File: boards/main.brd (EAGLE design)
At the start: 100 x 65 mm, 195 parts, among them IC1 24AA32ASN, IC2 INA194, IC3 LP2950Z, Q1 IRLML5203, Q2 IRLML5103, T3 BC848, U1 ITG-3200, U2 TMP75DGK, U3 MAG3110, U4 MMA8451Q, U44 BMP085, U5 MAX1236EUA+, X1 USB-SMD-NS

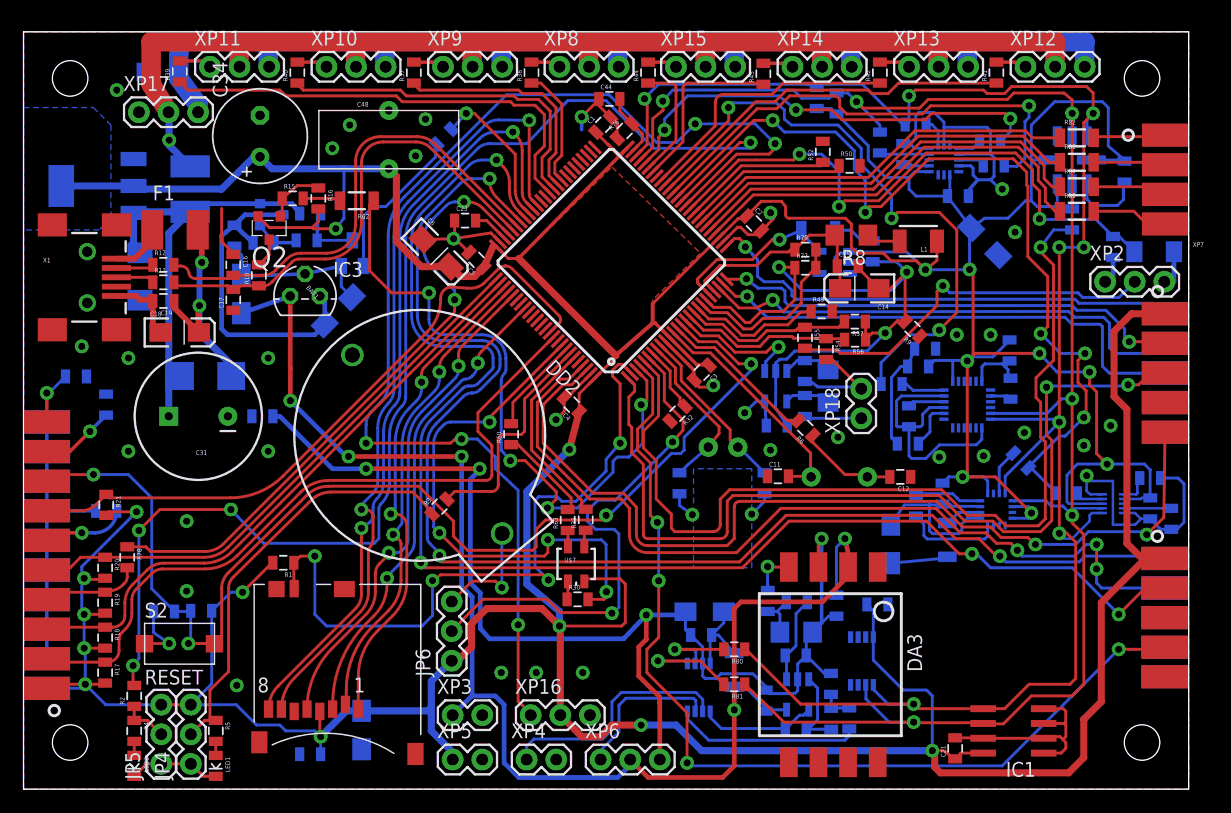
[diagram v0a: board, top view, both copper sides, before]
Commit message: put all the downloaded files into directories
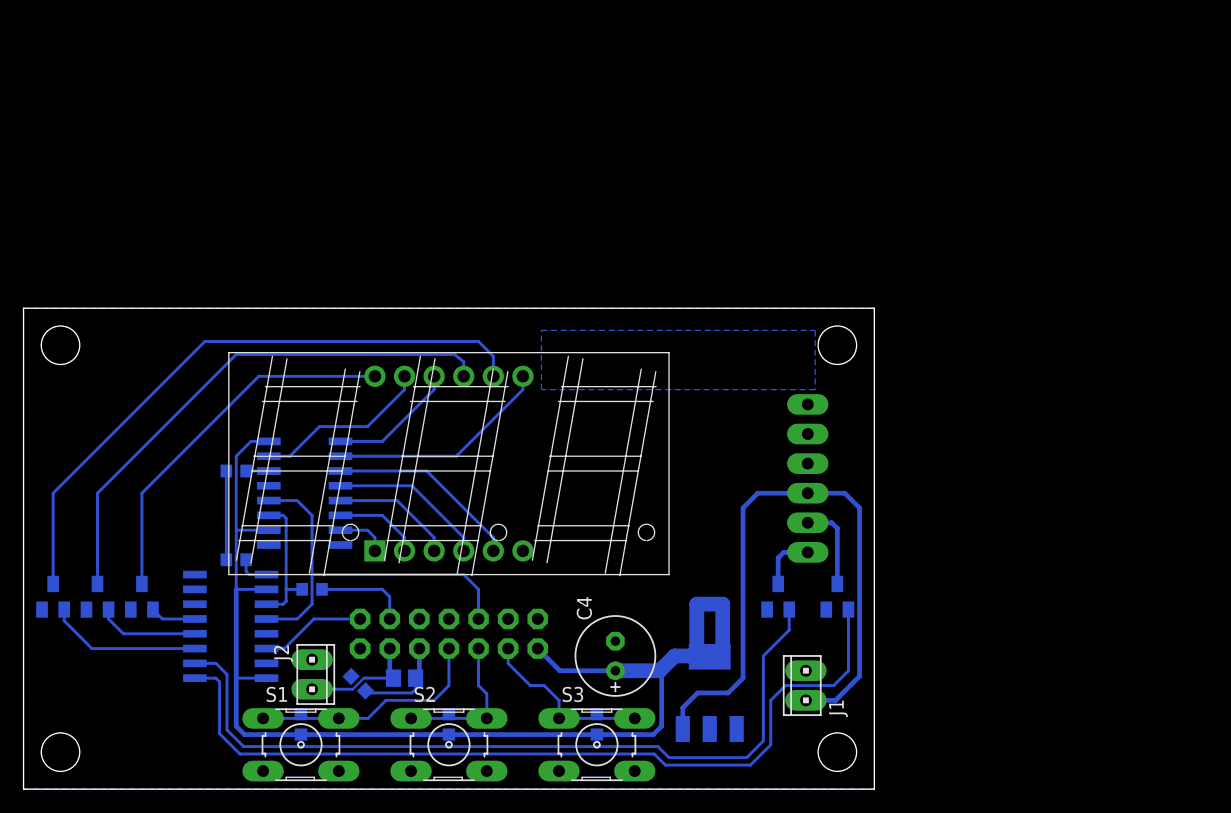
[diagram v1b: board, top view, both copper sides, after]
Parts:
- removed BAT1: 3V, SparkFun:BATTCOM_20MM_PTH
- removed C10, C9: 10pF, SparkFun:0805
- removed C11, C12, C16, C17: 20pF, SparkFun:0805
- removed C13, C15, C19, C20, C21, C22, C24, C25, C27, C28, C29, C32, C33, C36, C37, C38, C42, C43, C50, C54, C55, C8: 0.1uF, SparkFun:0805
- removed C14, C18, C52, C6: 10uF/6.3v, SparkFun:EIA3216-KIT
- removed C23, C44: 2.2uF, SparkFun:0805
- removed C26, C35, C41: 4.7uF, SparkFun:EIA3216-KIT
- removed C30: 1uF, SparkFun:0805
- removed C31: 330uF/16v, SparkFun:CPOL-RADIAL-1000UF-25V
- removed C34: 560uF/4v, rcl:E3,5-8
- removed C39: 2.2nF/50v, SparkFun:0805
- removed C40: 0.22uF, SparkFun:0805
- removed C45: 10uF, SparkFun:1206
- removed C48: 0.22F/5.5v, barthess:CAP-IONISTOR-5MM
- removed C49: 2.2uF, rcl:C1206
- removed C51: 10uF/16v, SparkFun:EIA3216-KIT
- removed C7: 47uF/6.3v, SparkFun:EIA3216-KIT
- removed D2: 10BQ060, diode:SMB
- removed D3: SM6T12V, diode:SMBJ
- removed DA1: LM1117, barthess:SOT223
- removed DA2: LMV321M5, linear:SOT23-5
- removed DA3: MPXV5010DP, barthess:482
- removed DA6: LP2980, barthess:SOT23-5
- removed DD1: MICROSD_SDIO, barthess:MICROSD
- removed DD2: STM32F103VDT6, barthess:TQFP100
- removed DD3: HMC5883L, barthess:16LPCC
- removed F1, F3: POLYSWITCH, barthess:1812
- removed IC2: INA194, barthess:SOT23-5
- removed JP1: 2X5, barthess:2X5-PSEUDOSMD
- removed JP3, JP7, JP8, JP9: STAND-OFFTIGHT, SparkFun:STAND-OFF-TIGHT
- removed JP4: boot_0, SparkFun:1X03
- removed JP5: boot_1, SparkFun:1X03
- removed JP6: bat, SparkFun:1X03
- removed L1: 1uH, SparkFun:1210
- removed LED1, LED2: RED, barthess:LED-0805
- removed R10, R35: 1.5k, SparkFun:0805
- removed R12, R13: 33, SparkFun:0805
- removed R15, R27, R28: 2.7k, SparkFun:0805
- removed R16, R17, R18, R19, R20, R21, R22, R23, R24, R45, R48, R54, R55, R59, R7: 10k, SparkFun:0805
- removed R25, R53: 2.2, barthess:R1206
- removed R26: 1, SparkFun:0805
- removed R29, R46, R56, R57, R58, R61, R66, R67, R69, R71, R72, R75: 1k, SparkFun:0805
- removed R30, R63: 68, SparkFun:0805
- removed R31, R60, R65, R70, R73, R74, R76, R77, R78, R79, R80, R81, R9: 0, SparkFun:0805
- removed R32, R33, R47: 100k, SparkFun:0805
- removed R34: 30k, SparkFun:0805
- removed R36, R51: 47, SparkFun:0805
- removed R37, R38, R39, R40, R41, R42, R43, R44, R49, R50, R52, R6: 330, SparkFun:0805
- removed R5: 100, SparkFun:0805
- removed R62, R64, R68, R82, R83, R84, R85: 0, barthess:R1206
- removed R8: 2.2, rcl:R1206
- removed T3: BC848, transistor:SOT23
- removed U$7: LED-TRICOLOR, SparkFun:LED-TRICOLOR-SMD
- removed U1: ITG-3200, barthess:QFN-24
- removed U2: TMP75DGK, barthess:MSOP8
- removed U3: MAG3110, barthess:DFN-10
- removed U4: MMA8451Q, barthess:QFN-16_0.5MM
- removed U44: BMP085, barthess:BMP085
- removed U5: MAX1236EUA+, barthess:MSOP8
- removed VD8: BZV55-C3V3, barthess:SOD80C
- removed X1: USB-SMD-NS, SparkFun:USB-MINIB-NOSTOP
- removed XP1: 2X10-PSEUDO_SMD, barthess:2X10-PSEUDOSMD
- removed XP10: PWM3, SparkFun:1X03
- removed XP11: PWM4, SparkFun:1X03
- removed XP12: PWM5, SparkFun:1X03
- removed XP13: PWM6, SparkFun:1X03
- removed XP14: PWM7, SparkFun:1X03
- removed XP15: PWM8, SparkFun:1X03
- removed XP16: tacho, SparkFun:1X03
- removed XP17: power, SparkFun:1X03
- removed XP18: current_sens, barthess:1X02
- removed XP2: RECEIVER, SparkFun:1X03
- removed XP3: EXT_5V, barthess:1X02
- removed XP4: an2_5v, barthess:1X02
- removed XP5: EXT3.3V, barthess:1X02
- removed XP6: sonar, SparkFun:1X03
- removed XP7: SPI_EXT, barthess:1X4-PSEUDOSMD
- removed XP8: PWM1, SparkFun:1X03
- removed XP9: PWM2, SparkFun:1X03
- removed ZQ1: 8M, barthess:HC49U-V
- removed ZQ2: 32k, barthess:TC38H
- added 430: (no value), pinhead:2X07
- added IC4: 74LS595D, 74xx-us:SO16
- added J1, J2: (no value), con-amp:10X02MTA
- added Q3, Q4, Q5: BSS123, transistor-small-signal:SOT23
- added S1, S3: (no value), switch-omron:B3F-10XX
- added U$1: BL-T52C-31, mjg:BL-T52X-31
- C1, C2, C3: value 0.1uF -> (none); device SparkFun:0805 -> rcl:C0603K
- C4: value 0.1uF -> (none); device SparkFun:0805 -> rcl:E2,5-7
- C5: value 0.1uF -> 470nF; device SparkFun:0805 -> rcl:C0603K
- IC1: value 24AA32ASN -> 74LS595D; device barthess:SO-08 -> 74xx-us:SO16
- IC3: value LP2950Z -> 317EMP; device linear:TO92 -> linear:SOT223
- JP2: value 2X5 -> (none); device barthess:2X5-PSEUDOSMD -> pinhead:1X06
- Q1: value IRLML5203 -> BSS123; device transistor-power:MICRO3 -> transistor-small-signal:SOT23
- Q2: value IRLML5103 -> BSS123; device transistor-power:MICRO3 -> transistor-small-signal:SOT23
- R1, R2: value 10k -> 0; device SparkFun:0805 -> rcl:R0603
- R3: value 10k -> 720ish; device SparkFun:0805 -> rcl:R0805
- R4: value 100 -> 0; device SparkFun:0805 -> rcl:R0603
- S2: value RESET -> (none); device barthess:BUTTON_6X3.5 -> switch-omron:B3F-10XX
- moved IC1 67.8 mm to (17.8, 14.0), flipped to the bottom
- moved C1 51.5 mm to (49.2, 5.56), flipped to the bottom, turned to 270 degrees
- moved C2 50.3 mm to (36.5, 5.56), flipped to the bottom, turned to 270 degrees
- moved IC3 48.7 mm to (58.9, 8.26), flipped to the bottom
- moved C3 45.8 mm to (23.8, 5.56), flipped to the bottom, turned to 270 degrees
- moved Q1 37.8 mm to (2.54, 16.5), turned to 0 degrees
- moved C5 37.8 mm to (28.7, 9.05), flipped to the bottom, turned to 225 degrees
- moved Q2 34.9 mm to (6.35, 16.5), flipped to the bottom, turned to 0 degrees
- moved JP2 32.9 mm to (67.3, 26.7), flipped to the bottom, turned to 270 degrees
- moved S2 28.1 mm to (36.5, 3.81)
- moved C4 21.9 mm to (50.8, 11.4), turned to 90 degrees
- moved R2 21.2 mm to (18.3, 27.3), flipped to the bottom, turned to 180 degrees
- moved R4 19.5 mm to (24.8, 17.1), flipped to the bottom, turned to 0 degrees
- moved R3 15.0 mm to (32.7, 9.53), flipped to the bottom, turned to 180 degrees
- moved R1 4.05 mm to (18.3, 19.7), flipped to the bottom, turned to 0 degrees
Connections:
- removed net 3.3V: C1.1, C2.1, C20.1, C21.1, C27.2, C3.1, C30.1, C33.2, C34.+, C35.A, C37.2, C4.1, C42.1, C48.1, C5.1, C6.A, C7.A, C8.2, DA1.2, DA1.4, DA6.1, DA6.3, DD1.4, DD2.100, DD2.11, DD2.28, DD2.50, DD2.75, DD3.13, DD3.2, DD3.4, IC1.8, JP1.1, JP2.1, JP4.3, JP5.3, JP6.1, L1.1, Q2.2, R1.2, R16.2, R17.2, R18.2, R19.2, R20.2, R21.2, R26.2, R27.2, R28.2, R7.2, U$7.A, U1.13, U2.8, U3.2, U3.8, U4.1, U4.14, U44.3, U44.4, U44.8, XP1.1, XP1.2, XP16.2, XP5.1
- removed net 5V: C24.1, C50.1, C52.A, DA2.5, DA3.2, IC3.1, R25.2, XP3.1, XP6.2
- removed net 5V_DOMAIN_ENABLE: DD2.67, R61.2
- removed net 5V_USB: C18.A, C19.1, D2.A, F1.2
- removed net 6V: C31.1, D2.C, D3.C, DA1.3, F3.2, Q1.2, R55.2, R59.1, XP2.2
- removed net AN3.3V_0: R49.2
- removed net AN3.3V_1: R50.2
- removed net AN3.3V_2: R52.2
- removed net AN5V_0: DA2.4, R33.2, U5.1
- removed net AN5V_1: U5.2, XP4.1
- removed net AN5V_2: U5.3, XP6.1
- removed net AN5V_3/REF: R34.2, U5.4
- removed net BMP085_EOC: DD2.5, R75.1
- removed net BOOT_0: DD2.94, R3.2
- removed net BOOT_1: DD2.37, R2.2
- removed net CURRENT_SENS: DD2.15, IC2.1
- removed net FROM_GPS: DD2.69, JP2.2
- removed net FROM_XBEE: DD2.26, JP1.2
- removed net GND_A: C14.C, C15.2, C22.2, C43.2, DA6.2, DD2.20, IC2.2, R56.1, R57.1, R77.1, R9.2
- removed net GND_A_5V: C24.2, C25.2, C26.C, C49.1, C50.2, DA2.2, DA3.3, R35.1, R47.1, R65.2, U5.7, XP6.3
- removed net GPS_ENABLE: DD2.4, JP2.7
- removed net GPS_PPS: DD2.97, JP2.4
- removed net I2C_SCL: DD2.47, DD3.1, IC1.6, R28.1, R73.1, R81.1, U1.23, U2.2, U3.7, U44.6
- removed net I2C_SDA: DD2.48, DD3.16, IC1.5, R27.1, R74.1, R80.1, U1.24, U2.1, U3.6, U44.7
- removed net ITG-3200_INT: DD2.41, R69.2
- removed net LED_B: DD2.95, R31.2
- removed net LED_G: DD2.93, R60.2
- removed net LED_R: DD2.92, R30.2
- removed net MAG_INT: DD2.38, R66.2, R67.1
- removed net MAIN_SUPPLY: R51.1, R54.2, XP18.2
- removed net MMA8451Q_INT1: DD2.39, R72.1
- removed net MMA8451Q_INT2: DD2.46, R71.1
- removed net N$27: C40.1, DD3.8
- removed net N$32: R29.1, XP2.1
- removed net N$33: R63.1, U$7.G
- removed net N$34: DD2.7, R32.1
- removed net N$35: C49.2, R46.2, R48.2
- removed net N$36: DD2.32, R82.1
- removed net N$37: C45.2, IC2.3, R51.2
- removed net N$38: C43.1, R53.1
- removed net N$39: R36.1, XP18.1
- removed net N$40: DD2.62, R39.1
- removed net N$41: DD2.61, R40.1
- removed net N$42: DD2.60, R37.1
- removed net N$43: DD2.59, R38.1
- removed net N$44: DA3.4, R46.1
- removed net N$45: DD2.34, R52.1
- removed net N$46: DA2.3, R33.1, R45.2
- removed net N$47: DA2.1, R47.2, R48.1
- removed net N$48: R34.1, R35.2, R45.1
- removed net N$49: DD2.33, R50.1
- removed net N$50: DD2.18, R49.1
- removed net N$51: DD2.31, R83.1
- removed net N$52: DD2.16, R54.1, R56.2
- removed net N$53: C54.1, Q1.1, R58.2
- removed net N$54: DD2.17, R55.1, R57.2
- removed net N$55: C51.A, C54.2, C55.1, IC3.3, Q1.3
- removed net N$56: R31.1, U$7.B
- removed net N$57: R30.1, U$7.R
- removed net N$58: DD2.30, R84.1
- removed net N$59: R61.1, T3.1
- removed net N$60: DD2.29, R85.1
- removed net N$61: DD2.45, R44.1
- removed net N$62: DD2.44, R43.1
- removed net N$63: DD2.42, R42.1
- removed net N$64: DD2.40, R41.1
- removed net N$65: R67.2, U3.9
- removed net N$66: DD3.15, R66.1
- removed net N$67: DD3.10, R68.1
- removed net N$68: R69.1, U1.12
- removed net N$69: R70.2, U1.8
- removed net N$70: R71.2, U4.9
- removed net N$71: R72.2, U4.11
- removed net N$72: R74.2, U4.6
- removed net N$73: R73.2, U4.4
- removed net N$74: R75.2, U44.2
- removed net N$75: R15.2, R62.2
- removed net N$76: R60.1, R63.2
- removed net N$77: R19.1, R78.2, XP1.7
- removed net N$78: R64.1, XP10.3, XP11.3, XP12.3, XP13.3, XP14.3, XP15.3, XP17.3, XP8.3, XP9.3
- removed net N$79: R80.2, U5.6
- removed net N$80: R81.2, U5.5
- removed net N$81: C23.2, DD2.73
- removed net N$82: C44.2, DD2.49, R76.2
- removed net N$83: DD2.19, R77.2, R79.2
- removed net NET$1: R58.1, R59.2, T3.3
- removed net PWM1: R38.2, XP8.1
- removed net PWM2: R37.2, XP9.1
- removed net PWM3: R40.2, XP10.1
- removed net PWM4: R39.2, XP11.1
- removed net PWM5: R41.2, XP12.1
- removed net PWM6: R42.2, XP13.1
- removed net PWM7: R43.2, XP14.1
- removed net PWM8: R44.2, XP15.1
- removed net RECEIVER_PPM: DD2.35, R29.2, VD8.C
- removed net RESET: C13.1, DD2.14, R7.1, S2.S, XP1.15
- removed net SDIO_CK: DD1.5, DD2.80
- removed net SDIO_CMD: DD1.3, DD2.83
- removed net SDIO_D0: DD1.7, DD2.65
- removed net SDIO_D1: DD1.8, DD2.66
- removed net SDIO_D2: DD1.1, DD2.78
- removed net SDIO_D3: DD1.2, DD2.79
- removed net SDIO_DETECT: DD1.13, DD2.2, R1.1
- removed net SPI_EXT_MISO: R83.2, XP7.2
- removed net SPI_EXT_MOSI: R82.2, XP7.1
- removed net SPI_EXT_NSS: R85.2, XP7.4
- removed net SPI_EXT_SCK: R84.2, XP7.3
- removed net TACHOMETER: DD2.36, XP16.1
- removed net TCK: DD2.76, R20.1, XP1.9
- removed net TDI: DD2.77, R18.1, XP1.5
- removed net TDO: DD2.89, R21.1, XP1.13
- removed net TMP75_ALERT: U2.3
- removed net TMS: DD2.72, R78.1
- removed net TO_GPS: DD2.68, JP2.3
- removed net TO_XBEE: DD2.25, JP1.3
- removed net TRST: DD2.90, R17.1, XP1.3
- removed net USB_DISCOVERY: DD2.3, R62.1
- removed net USB_DM: C16.2, DD2.70, R12.2
- removed net USB_DP: C17.2, DD2.71, R10.1, R13.2
- removed net VBAT: DD2.6, JP6.2
- removed net VDD_A: C14.A, C15.1, C22.1, DD2.22, IC2.5, R79.1, R8.2
- removed net VREF_MCU: DA6.5, DD2.21, R53.2
- removed net V_IN: F3.1, XP10.2, XP11.2, XP12.2, XP13.2, XP14.2, XP15.2, XP17.2, XP8.2, XP9.2
- removed net XBEE_CTS: DD2.23, JP1.4
- removed net XBEE_RESET: DD2.1, JP1.5
- removed net XBEE_RTS: DD2.24, JP1.6
- removed net XBEE_SLEEP: DD2.98, JP1.9
- new net +5V: IC3.3, J1.2, JP2.4
- new net N$15: 430.7, C3.1, S1.1, S1.2
- new net VCC: 430.1, C1.2, C2.2, C3.2, C4.+, IC1.10, IC1.16, IC3.4, IC4.10, IC4.16
- net GND: now also 430.13, 430.2, C4.-, C5.1, IC1.13, IC1.8, IC3.1, IC4.13, IC4.8, J1.1, J2.2, JP2.2, JP2.3, Q1.2, Q2.2, Q3.2, Q4.2, Q5.2, S1.3, S1.4, S2.3, S2.4, S3.3, S3.4; no longer BAT1.2, C1.2, C10.2, C11.1, C12.1, C13.2, C16.1, C17.1, C18.C, C19.2, C2.2, C20.2, C21.2, C23.1, C27.1, C28.1, C29.1, C3.2, C30.2, C31.2, C32.1, C33.1, C34.-, C35.C, C36.1, C37.1, C38.1, C39.1, C4.2, C41.C, C42.2, C44.1, C48.2, C5.2, C51.C, C52.C, C55.2, C6.C, C7.C, C8.1, C9.2, D3.A, DA1.1, DD1.10, DD1.11, DD1.12, DD1.6, DD1.9, DD2.10, DD2.27, DD2.74, DD2.99, DD3.11, DD3.9, IC1.1, IC1.2, IC1.3, IC1.4, IC1.7, IC3.2, JP1.10, JP2.10, JP4.1, JP5.1, LED1.C, LED2.C, R22.1, R23.1, R24.1, R32.2, R64.2, R65.1, R76.1, R9.1, S2.P, T3.2, U1.1, U1.11, U1.18, U1.9, U2.4, U2.5, U2.6, U2.7, U3.10, U3.5, U4.10, U4.12, U4.5, U4.7, U44.1, VD8.A, X1.GND, XP1.10, XP1.12, XP1.14, XP1.16, XP1.18, XP1.20, XP1.4, XP1.6, XP1.8, XP16.3, XP2.3, XP3.2, XP4.2, XP5.2
- net N$1: now also IC4.15, U$1.P$8; no longer C9.1, DD2.9, ZQ2.2
- net N$10: now also Q2.3, U$1.P$10; no longer R12.1, X1.D-
- net N$11: now also Q3.3, U$1.P$7; no longer BAT1.1, JP6.3
- net N$12: now also IC1.3, Q1.1; no longer L1.2, R8.1
- net N$13: now also 430.14, IC1.14; no longer R13.1, X1.D+
- net N$14: now also IC4.14, R2.2; no longer Q2.3, R10.2
- net N$16: now also IC1.9, R1.1; no longer Q2.1, R15.1, R16.1
- net N$17: now also 430.11, J2.1, JP2.1, R3.1; no longer R22.2, XP1.19
- net N$18: now also 430.3, C1.1, S3.1, S3.2; no longer R23.2, XP1.17
- net N$19: now also R1.2, R2.1; no longer R24.2, XP1.11
- net N$2: now also IC4.1, U$1.P$9; no longer LED2.A, R4.2
- net N$20: now also IC1.1, Q4.1; no longer C45.1, IC2.4, R36.2
- net N$21: now also IC1.11, IC4.11, R4.2; no longer C25.1, C26.A, R25.1, U5.8
- net N$22: now also IC1.4, Q2.1; no longer C32.2, U4.2
- net N$23: now also JP2.5, Q4.3; no longer C36.2, U1.10
- net N$24: now also IC1.5, Q3.1; no longer C29.2, U3.4
- net N$25: now also IC1.2, Q5.1; no longer C38.2, R26.1, R70.1
- net N$26: now also 430.12, R4.1; no longer C28.2, U3.1
- net N$28: now also JP2.6, Q5.3; no longer C40.2, DD3.12
- net N$29: now also 430.5, C2.1, S2.1, S2.2; no longer F1.1, X1.VBUS
- net N$3: now also IC4.7, U$1.P$1; no longer JP5.2, R2.1, R4.1
- net N$30: now also 430.6, IC1.12, IC4.12; no longer C39.2, U1.20
- net N$31: now also 430.9, C5.2, R3.2; no longer C41.A, R68.2
- net N$4: now also IC4.6, U$1.P$2; no longer LED1.A, R5.2
- net N$5: now also IC4.5, U$1.P$3; no longer JP4.2, R3.1, R5.1
- net N$6: now also IC4.4, U$1.P$4; no longer C10.1, DD2.8, ZQ2.1
- net N$7: now also IC4.3, U$1.P$5; no longer DD2.13, R6.2
- net N$8: now also IC4.2, U$1.P$12; no longer C12.2, R6.1, ZQ1.2
- net N$9: now also Q1.3, U$1.P$11; no longer C11.2, DD2.12, ZQ1.1
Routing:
- net 3.3V: track 574.1 -> 0.00 mm, vias 20 -> 0
- net GND: track 228.1 -> 0.00 mm, vias 36 -> 0
- net I2C_SDA: track 161.2 -> 0.00 mm, vias 8 -> 0
- net I2C_SCL: track 153.4 -> 0.00 mm, vias 6 -> 0
- net 5V: track 124.3 -> 0.00 mm, vias 5 -> 0
- net TO_GPS: track 121.8 -> 0.00 mm, vias 4 -> 0
- net FROM_GPS: track 115.1 -> 0.00 mm, vias 3 -> 0
- net BOOT_1: track 108.4 -> 0.00 mm, vias 4 -> 0
- net V_IN: track 106.8 -> 0.00 mm, vias 1 -> 0
- net TACHOMETER: track 105.8 -> 0.00 mm, vias 5 -> 0
- net VCC: track 0.00 -> 105.3 mm
- net GND_A_5V: track 103.9 -> 0.00 mm, vias 4 -> 0
- net N$78: track 102.4 -> 0.00 mm
- net RESET: track 100.3 -> 0.00 mm, vias 4 -> 0
- net GPS_ENABLE: track 83.0 -> 0.00 mm, vias 4 -> 0
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- added copper zone on layer 16, net N$27
- added copper zone on layer 16, net VCC
- removed copper zone on layer 1, net 3.3V
- removed copper zone on layer 16, net 3.3V
- removed copper zone on layer 1, net GND
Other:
- board size 100 x 65 mm -> 73 x 41.3 mm
- board text added: "2012 Matthew Gardeski"
- board text added: "FUSERATOR V6"
